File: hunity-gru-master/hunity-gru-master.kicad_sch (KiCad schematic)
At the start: 12 parts, among them J1 Conn_01x10_Pin, J2 Conn_01x10_Socket, U1 BME280, U2 AP2112K-3.3

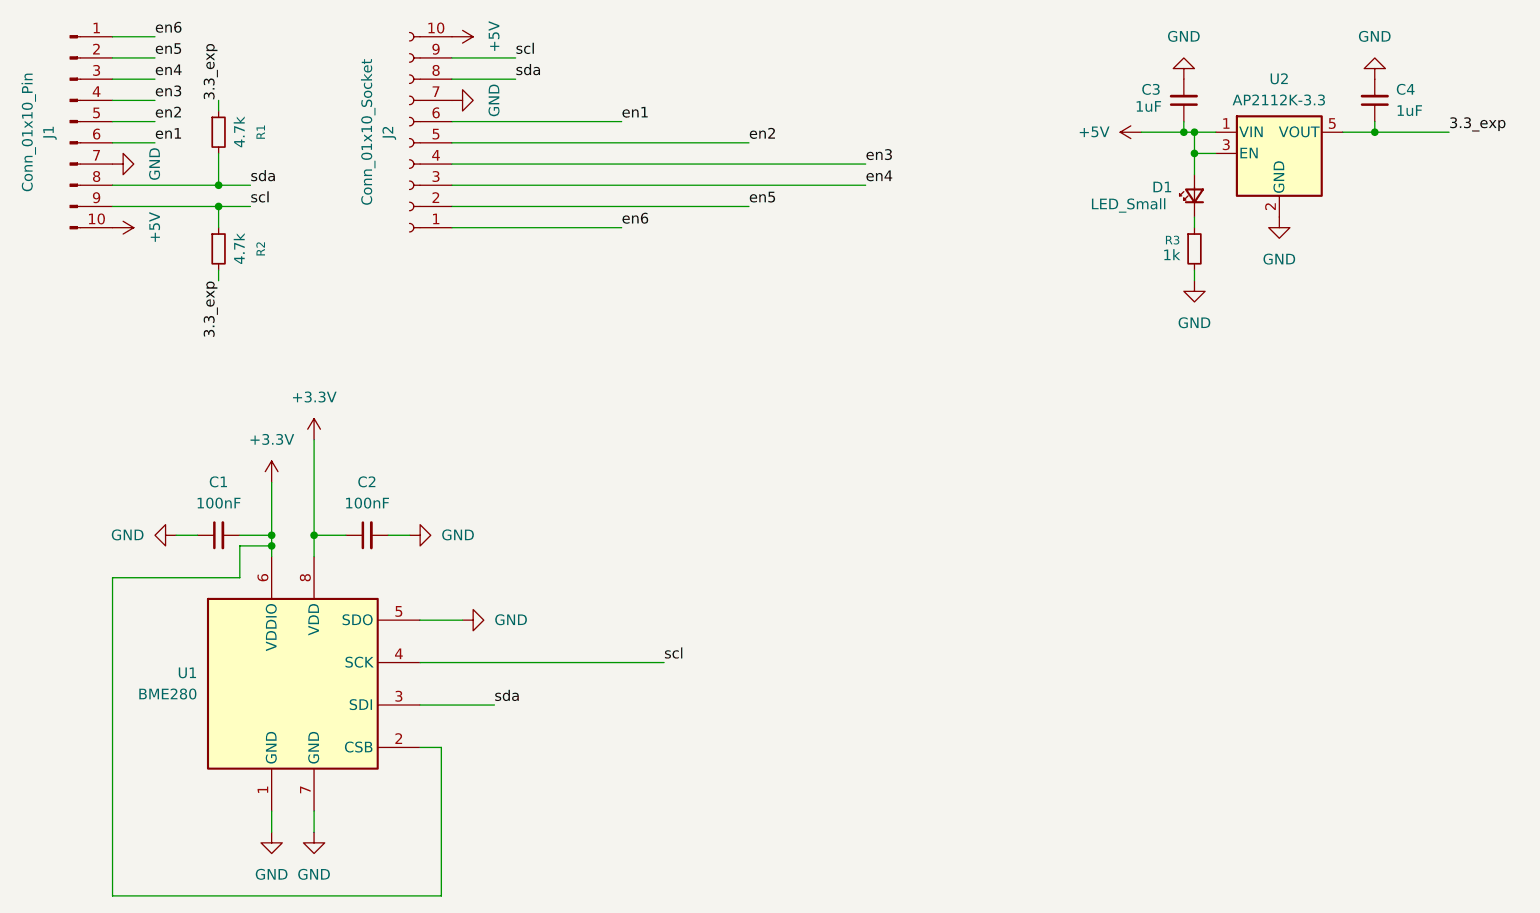
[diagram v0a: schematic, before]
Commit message: idk
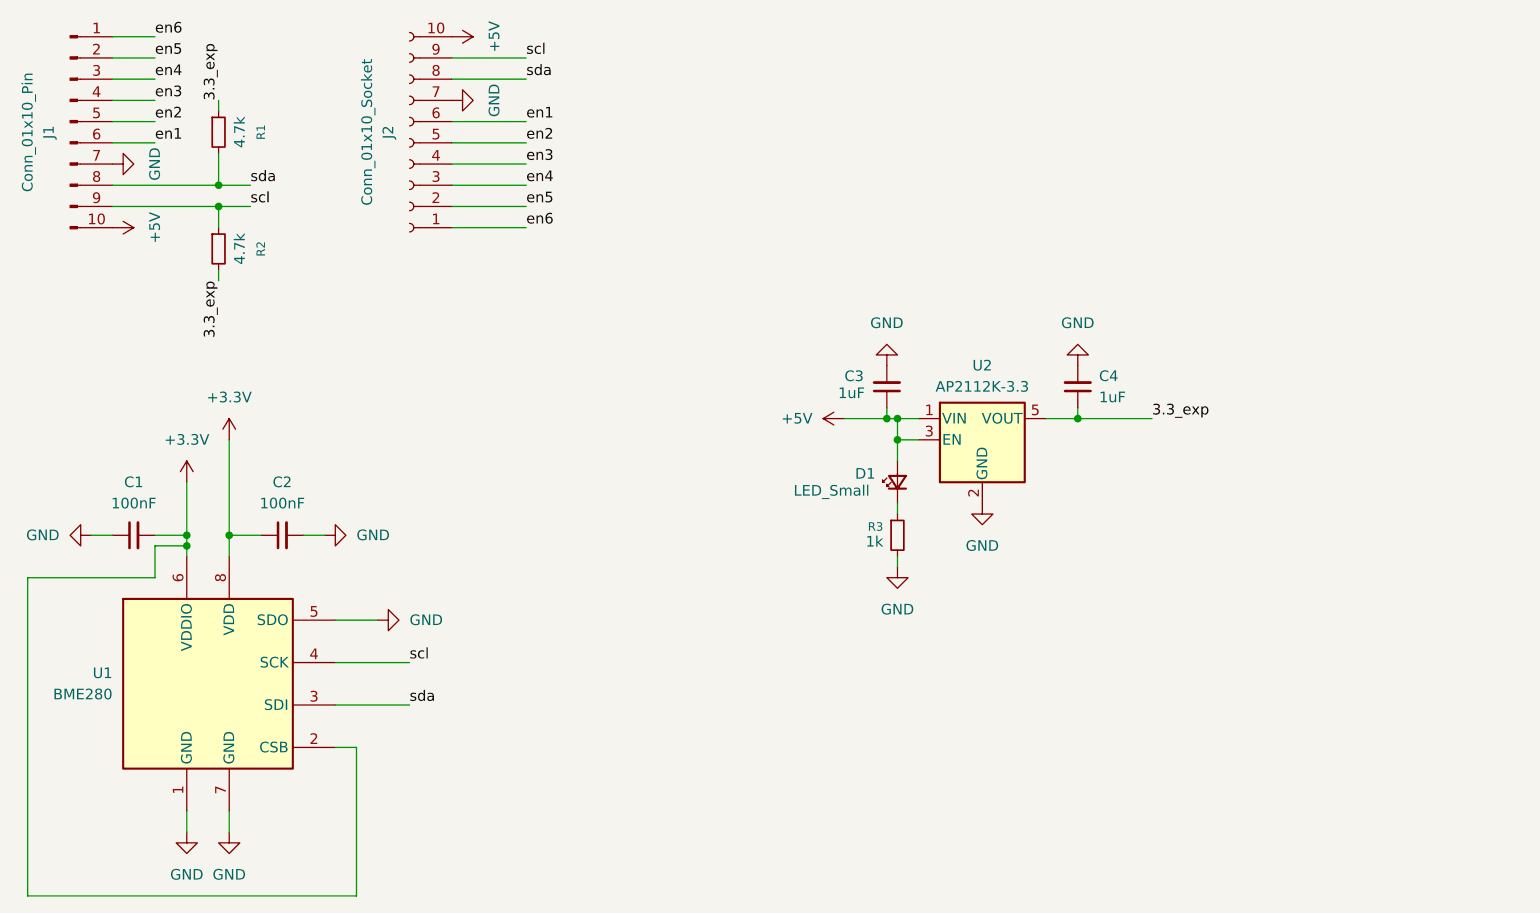
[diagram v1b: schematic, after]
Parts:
- J1: footprint Connector_PinHeader_2.54mm:PinHeader_1x10_P2.54mm_Horizontal -> hunity_gru_temp:header
- J2: footprint Connector_PinSocket_2.54mm:PinSocket_1x10_P2.54mm_Horizontal -> hunity_gru_temp:socket
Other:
- company: (none) -> OnionSAT
- title: (none) -> Hunity GRU 
- moved on the sheet: C1, C2, C3, C4, D1, R3, U1, U2
